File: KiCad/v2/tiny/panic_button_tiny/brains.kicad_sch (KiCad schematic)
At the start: 24 parts, among them J3 PINHD_1x6_Male, SW1 Switch_Tactile_CnK, SW2 Switch_Tactile_CnK, SW3 Switch_Tactile_CnK, U5 ESP32-C3, Y1 C3E40000121010X, Y2 CTS3-32.768-12.5-20-R

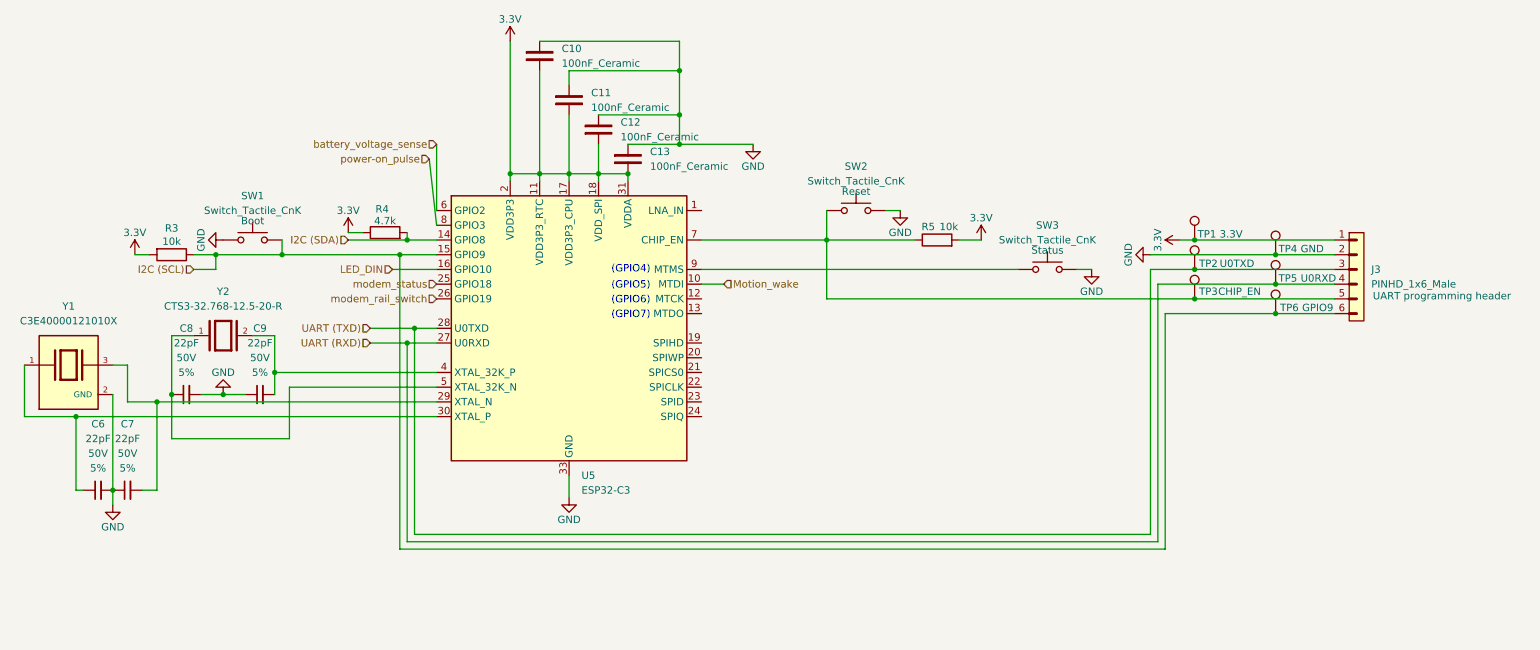
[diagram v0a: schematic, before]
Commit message: [UPDATE] the schematic wirering
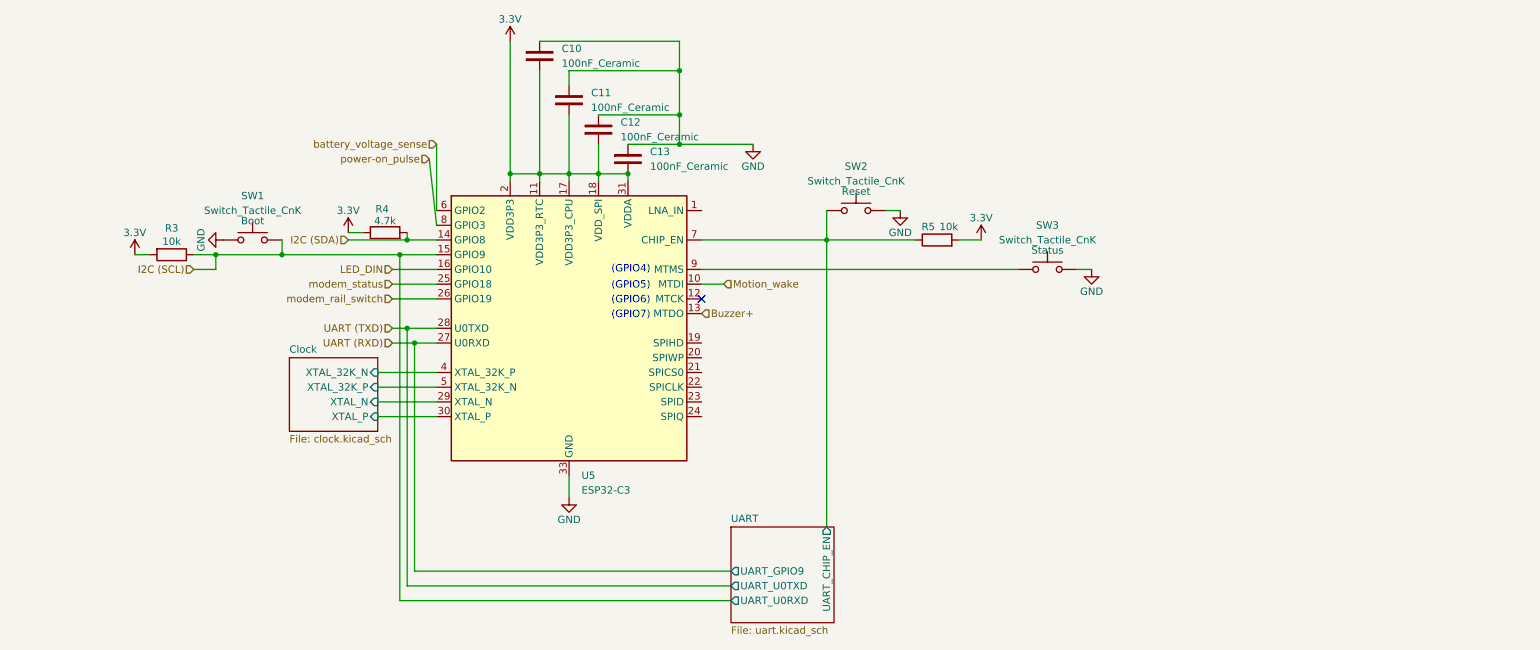
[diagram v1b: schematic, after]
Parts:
- removed C6, C7, C8, C9: 22pF, PCM_SparkFun-Capacitor:C_0402_1005Metric, symbol PCM_SparkFun-Capacitor:22pF_0402_50V_5%
- removed J3: PINHD_1x6_Male, Connector_PinHeader_2.54mm:PinHeader_1x06_P2.54mm_Vertical, symbol PCM_SL_Pin_Headers:PINHD_1x6_Male
- removed TP1: 3.3V, TestPoint:TestPoint_Pad_D4.0mm, symbol Connector:TestPoint
- removed TP2: U0TXD, TestPoint:TestPoint_Pad_D4.0mm, symbol Connector:TestPoint
- removed TP3: CHIP_EN, TestPoint:TestPoint_Pad_D4.0mm, symbol Connector:TestPoint
- removed TP4: GND, TestPoint:TestPoint_Pad_D4.0mm, symbol Connector:TestPoint
- removed TP5: U0RXD, TestPoint:TestPoint_Pad_D4.0mm, symbol Connector:TestPoint
- removed TP6: GPIO9, TestPoint:TestPoint_Pad_D4.0mm, symbol Connector:TestPoint
- removed Y1: C3E40000121010X, C3E40000121010X:XTAL_C3E40000121010X, symbol C3E40000121010X:C3E40000121010X
- removed Y2: CTS3-32.768-12.5-20-R, CTS3-32.768-12.5-20-R:XTAL_CTS3-32.768-12.5-20-R, symbol CTS3-32.768-12.5-20-R:CTS3-32.768-12.5-20-R
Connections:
- net Clock/XTAL_N: now reaches U5.29 (XTAL_N)
- net Clock/XTAL_P: now reaches U5.30 (XTAL_P)
- net UART/UART_CHIP_EN: now reaches R5.1, SW2.1, U5.7 (CHIP_EN)
- net Clock/XTAL_32K_P: now reaches U5.5 (XTAL_32K_N)
- net Clock/XTAL_32K_N: now reaches U5.4 (XTAL_32K_P)
- net Buzzer+: now reaches U5.13 (MTDO)
- no-connect marks 0 -> 1
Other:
- added sheet Clock (clock.kicad_sch)
- added sheet UART (uart.kicad_sch)
